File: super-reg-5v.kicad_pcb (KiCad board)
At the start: 2 copper layers, 80 x 33 mm, 39 parts, among them Q1 2SA1015, Q2 D44H11, U1 LM317T, U2 AD825, X1 AC_IN, X2 DC_OUT

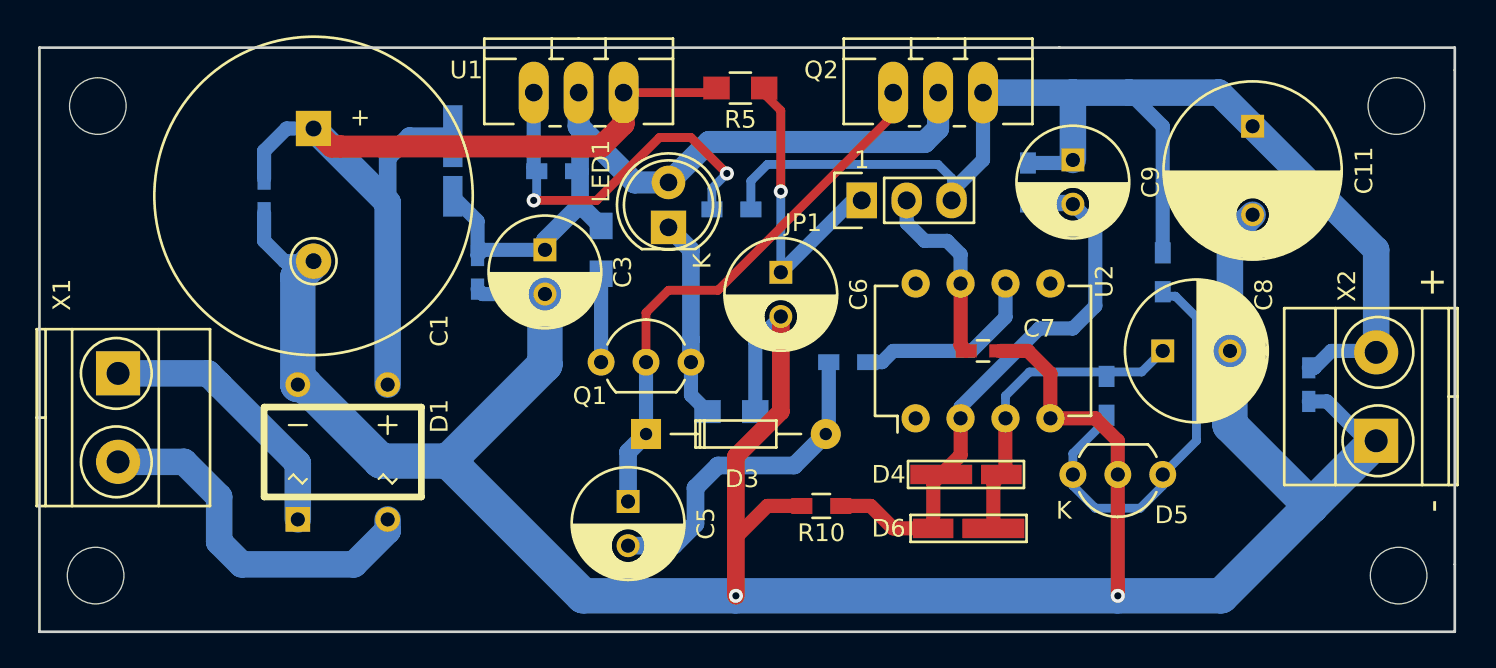
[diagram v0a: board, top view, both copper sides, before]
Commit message: minor track fix
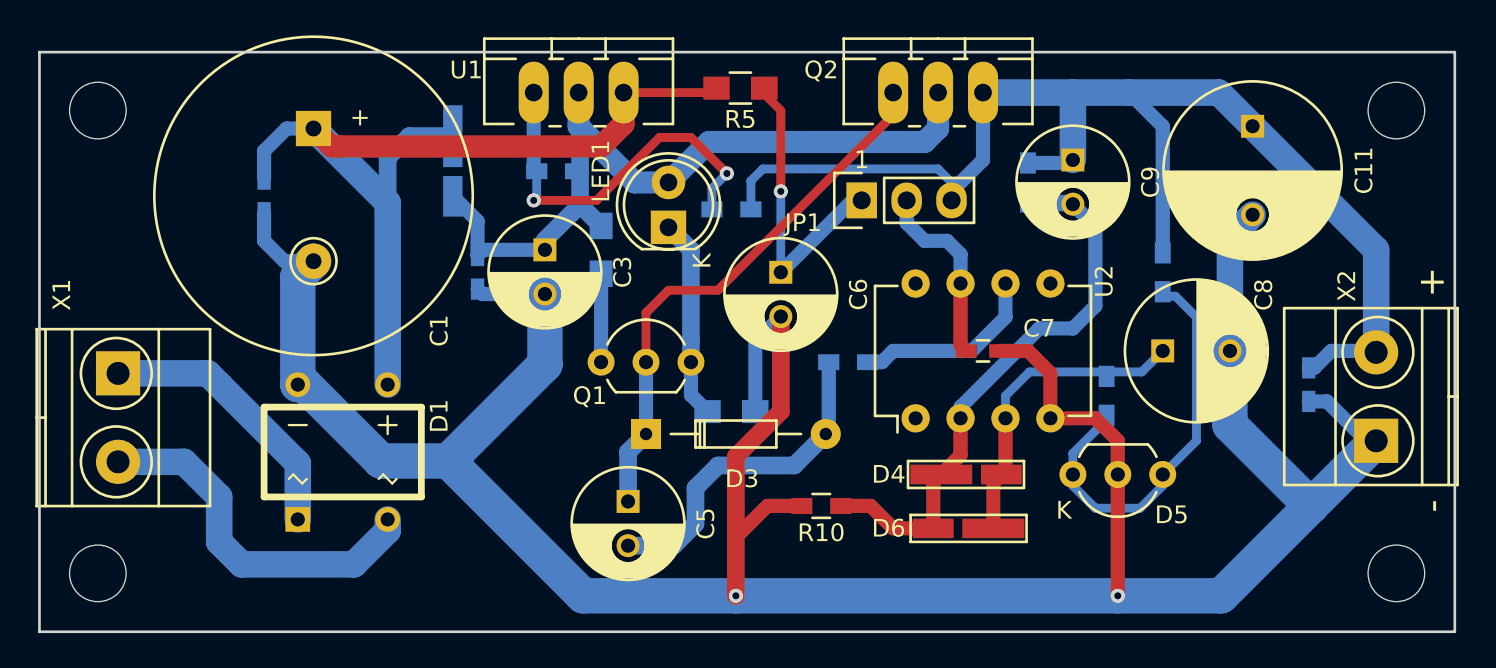
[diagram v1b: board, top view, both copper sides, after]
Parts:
- moved ? 0.25 mm to (192.3, 77.2)
- moved REF** 0.25 mm to (118.9, 77.2)
- moved REF** 0.18 mm to (192.3, 103.4)
- moved REF** 0.18 mm to (118.9, 103.4)
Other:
- board size 80 x 33 mm -> 80 x 32.8 mm
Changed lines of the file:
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@@
     (links 63)
     (no_connects 0)
-    (area 106.014857 68.802 205.262143 110.245)
+    (area 106.014857 69.056 205.135143 110.118)
     (thickness 1.6)
-    (drawings 11)
+    (drawings 8)
     (tracks 199)
     (zones 0)
@@
   )
   (setup
-    (last_trace_width 0.8)
+    (last_trace_width 0.25)
     (user_trace_width 0.25)
     (user_trace_width 0.5)
@@
     (pad_to_mask_clearance 0.2)
     (aux_axis_origin 0 0)
+    (grid_origin 115.57 73.914)
     (visible_elements FFFFFF7F)
     (pcbplotparams
-      (layerselection 0x00030_80000001)
-      (usegerberextensions false)
+      (layerselection 0x010f0_80000001)
+      (usegerberextensions true)
       (excludeedgelayer true)
       (linewidth 0.100000)
@@
       (psa4output false)
       (plotreference true)
-      (plotvalue true)
+      (plotvalue false)
       (plotinvisibletext false)
       (padsonsilk false)
-      (subtractmaskfromsilk false)
+      (subtractmaskfromsilk true)
       (outputformat 1)
       (mirror false)
       (drillshape 0)
       (scaleselection 1)
-      (outputdirectory ""))
+      (outputdirectory gerber/))
   )
   (net 0 "")
@@
   )
   (module Mounting_Holes:MountingHole_3.2mm_M3 (layer F.Cu)
-    (at 118.745 103.505)
+    (at 118.872 103.378)
     (descr "Mounting Hole 3.2mm, no annular, M3")
     (tags "mounting hole 3.2mm no annular m3")
@@
   )
   (module Mounting_Holes:MountingHole_3.2mm_M3 (layer F.Cu)
-    (at 192.405 103.505)
+    (at 192.278 103.378)
     (descr "Mounting Hole 3.2mm, no annular, M3")
     (tags "mounting hole 3.2mm no annular m3")
@@
   )
   (module Mounting_Holes:MountingHole_3.2mm_M3 (layer F.Cu)
-    (at 118.872 76.962)
+    (at 118.872 77.216)
     (descr "Mounting Hole 3.2mm, no annular, M3")
     (tags "mounting hole 3.2mm no annular m3")
@@
   )
   (module Mounting_Holes:MountingHole_3.2mm_M3 (layer F.Cu)
-    (at 192.278 76.962)
+    (at 192.278 77.216)
     (descr "Mounting Hole 3.2mm, no annular, M3")
     (tags "mounting hole 3.2mm no annular m3")
@@
     )
   )
+  (gr_line (start 195.58 73.914) (end 195.58 106.68) (angle 90) (layer Edge.Cuts) (width 0.15))
+  (gr_line (start 115.57 73.914) (end 115.57 106.68) (angle 90) (layer Edge.Cuts) (width 0.15))
+  (gr_line (start 195.58 73.914) (end 115.57 73.914) (angle 90) (layer Edge.Cuts) (width 0.15))
   (gr_text 1 (at 162.052 80.01) (layer F.SilkS)
     (effects (font (size 1 1) (thickness 0.15)))
@@
     (effects (font (size 1 1) (thickness 0.15)))
   )
-  (gr_line (start 173.228 73.66) (end 195.58 73.66) (angle 90) (layer Edge.Cuts) (width 0.15))
-  (gr_line (start 115.57 106.68) (end 115.57 73.66) (angle 90) (layer Edge.Cuts) (width 0.15))
-  (gr_line (start 173.228 73.66) (end 115.57 73.66) (angle 90) (layer Edge.Cuts) (width 0.15))
   (gr_text - (at 194.31 99.568 90) (layer F.SilkS)
     (effects (font (size 1.5 1.5) (thickness 0.3)))
@@
     (effects (font (size 1.5 1.5) (thickness 0.3)))
   )
-  (gr_line (start 195.58 106.68) (end 195.58 102.87) (angle 90) (layer Edge.Cuts) (width 0.15))
   (gr_line (start 115.57 106.68) (end 195.58 106.68) (angle 90) (layer Edge.Cuts) (width 0.15))
-  (gr_line (start 195.58 74.93) (end 195.58 73.66) (angle 90) (layer Edge.Cuts) (width 0.15))
-  (gr_line (start 195.58 102.87) (end 195.58 74.93) (angle 90) (layer Edge.Cuts) (width 0.15))
   (segment (start 135.255 82.55) (end 135.255 79.883) (width 1) (layer B.Cu) (net 1))
   (segment (start 136.474 78.664) (end 138.938 78.664) (width 1) (layer B.Cu) (net 1))
@@
   (segment (start 153.59 76.2) (end 153.844 75.946) (width 0.5) (layer F.Cu) (net 1))
   (segment (start 138.862 78.74) (end 138.938 78.664) (width 0.8) (layer B.Cu) (net 1))
-  (segment (start 156.036 94.234) (end 156.036 90.304) (width 0.8) (layer B.Cu) (net 2) (status 400000))
-  (segment (start 156.036 90.304) (end 157.48 88.86) (width 0.8) (layer B.Cu) (net 2) (status 800000))
+  (segment (start 156.036 94.234) (end 156.036 90.304) (width 0.8) (layer B.Cu) (net 2))
+  (segment (start 156.036 90.304) (end 157.48 88.86) (width 0.8) (layer B.Cu) (net 2))
   (segment (start 154.94 104.648) (end 154.94 96.774) (width 1) (layer F.Cu) (net 2))
-  (segment (start 157.48 94.234) (end 157.48 88.86) (width 1) (layer F.Cu) (net 2) (status 800000))
+  (segment (start 157.48 94.234) (end 157.48 88.86) (width 1) (layer F.Cu) (net 2))
   (segment (start 154.94 96.774) (end 157.48 94.234) (width 1) (layer F.Cu) (net 2))
   (segment (start 158.666 99.568) (end 156.718 99.568) (width 0.8) (layer F.Cu) (net 2))
@@
   (segment (start 154.94 101.346) (end 154.94 104.648) (width 0.8) (layer F.Cu) (net 2))
   (segment (start 176.53 97.79) (end 176.53 104.648) (width 0.8) (layer F.Cu) (net 2))
-  (via (at 176.53 104.648) (size 0.8) (drill 0.4) (layers F.Cu B.Cu) (net 2) (status 1000000))
+  (via (at 176.53 104.648) (size 0.8) (drill 0.4) (layers F.Cu B.Cu) (net 2))
   (segment (start 182.87 90.805) (end 182.87 94.986) (width 2) (layer B.Cu) (net 2))
   (segment (start 182.87 94.986) (end 187.452 99.568) (width 2) (layer B.Cu) (net 2))
@@
   (segment (start 170.18 93.345) (end 171.53 91.995) (width 0.5) (layer B.Cu) (net 7))
   (segment (start 171.53 91.995) (end 175.895 91.995) (width 0.5) (layer B.Cu) (net 7))
-  (segment (start 155.786 82.804) (end 155.786 81.196) (width 0.5) (layer B.Cu) (net 8))
-  (segment (start 167.132 81.026) (end 167.132 82.296) (width 0.5) (layer B.Cu) (net 8))
-  (segment (start 166.37 80.264) (end 167.132 81.026) (width 0.5) (layer B.Cu) (net 8))
-  (segment (start 156.718 80.264) (end 166.37 80.264) (width 0.5) (layer B.Cu) (net 8))
-  (segment (start 155.786 81.196) (end 156.718 80.264) (width 0.5) (layer B.Cu) (net 8))
+  (segment (start 167.132 82.296) (end 167.132 81.28) (width 0.5) (layer B.Cu) (net 8))
+  (segment (start 167.132 81.28) (end 166.37 80.518) (width 0.5) (layer B.Cu) (net 8))
+  (segment (start 166.37 80.518) (end 156.464 80.518) (width 0.5) (layer B.Cu) (net 8))
+  (segment (start 156.464 80.518) (end 155.786 81.196) (width 0.5) (layer B.Cu) (net 8))
+  (segment (start 155.786 81.196) (end 155.786 82.804) (width 0.5) (layer B.Cu) (net 8))
   (segment (start 168.91 76.2) (end 168.91 80.01) (width 0.8) (layer B.Cu) (net 8))
   (segment (start 168.91 80.01) (end 167.132 81.788) (width 0.8) (layer B.Cu) (net 8))
